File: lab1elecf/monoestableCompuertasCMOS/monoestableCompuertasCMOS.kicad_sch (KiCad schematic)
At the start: 10 parts, among them J1 Conn_01x02, J2 Conn_01x02, J3 Conn_01x02, J4 Conn_01x02, U1 74AUC2G02, U2 74AHC2G00

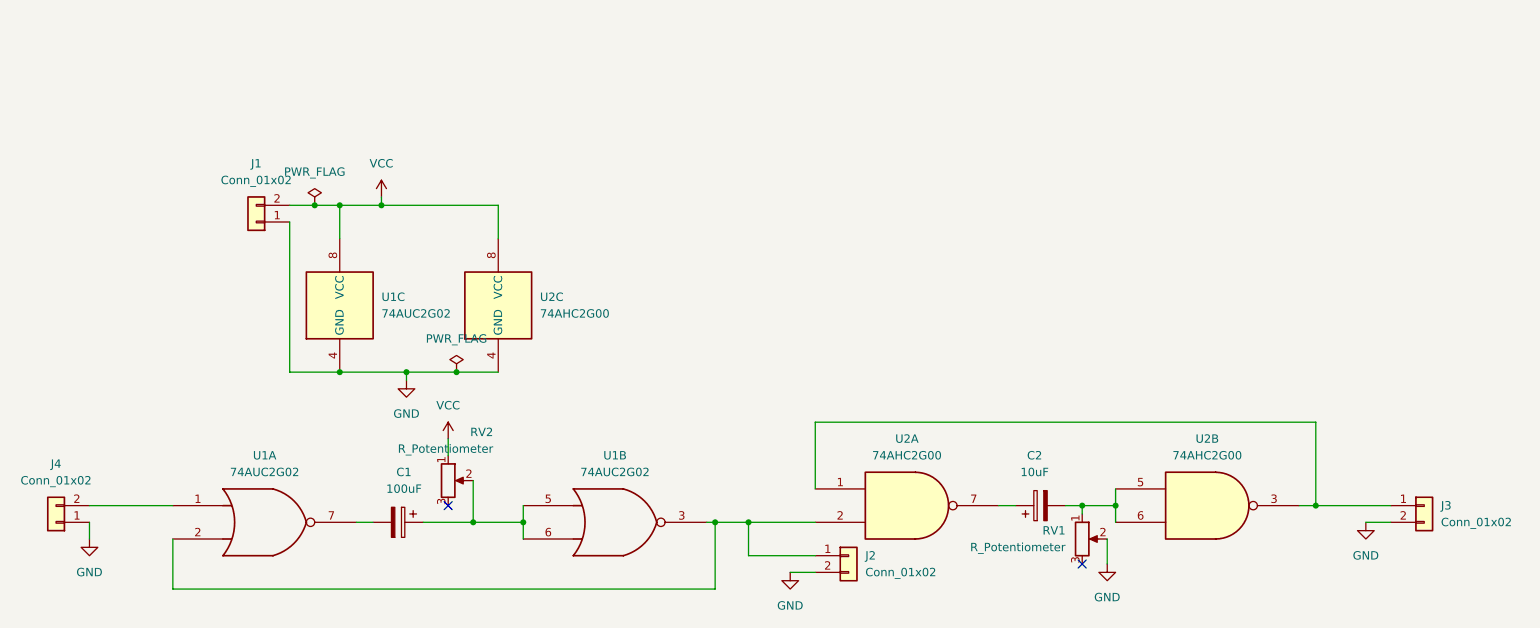
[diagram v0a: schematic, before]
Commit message: monoCMOS nefasto
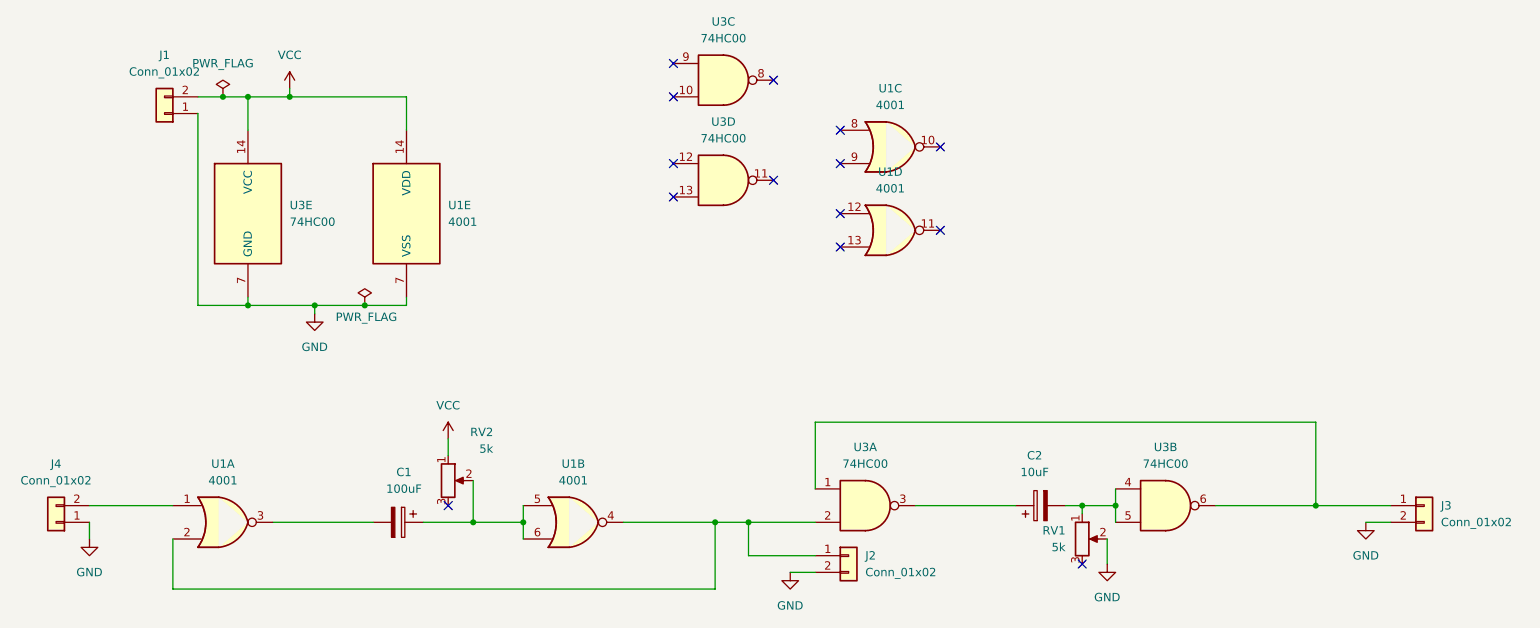
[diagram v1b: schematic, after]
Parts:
- removed U1: 74AUC2G02, symbol 74xGxx:74AUC2G02
- removed U2: 74AHC2G00, symbol 74xGxx:74AHC2G00
- added U1: 4001, Package_DIP:DIP-14_W7.62mm_Socket, symbol 4xxx:4001
- added U3: 74HC00, Package_DIP:DIP-14_W7.62mm_Socket, symbol 74xx:74HC00
- RV1, RV2: value R_Potentiometer -> 5k; footprint (none) -> Potentiometer_THT:Potentiometer_Alps_RK163_Single_Horizontal
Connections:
- net GND: now also U1.7 (VSS), U3.7 (GND)
- net VCC: now also U1.14 (VDD), U3.14 (VCC)
- net at C1.1, RV2.2: now also U1.5, U1.6
- net at J3.1 (Pin_1): now also U3.1, U3.6
- net at C2.2, RV1.1: now also U3.4, U3.5
- net at C1.2: now also U1.3
- net at J2.1 (Pin_1): now also U1.2, U1.4, U3.2
- net at C2.1: now also U3.3
- net at J4.2 (Pin_2): now also U1.1
- no-connect marks 2 -> 14
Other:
- moved on the sheet: J1
